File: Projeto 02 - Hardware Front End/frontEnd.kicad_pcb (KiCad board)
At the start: 2 copper layers, 75 x 50 mm, 22 parts, among them J1 Power_Supply, J2 Signal_Input, J3 MCU_Interface, U1 L78L12_TO92, U2 L79L12_TO92, U3 LM311

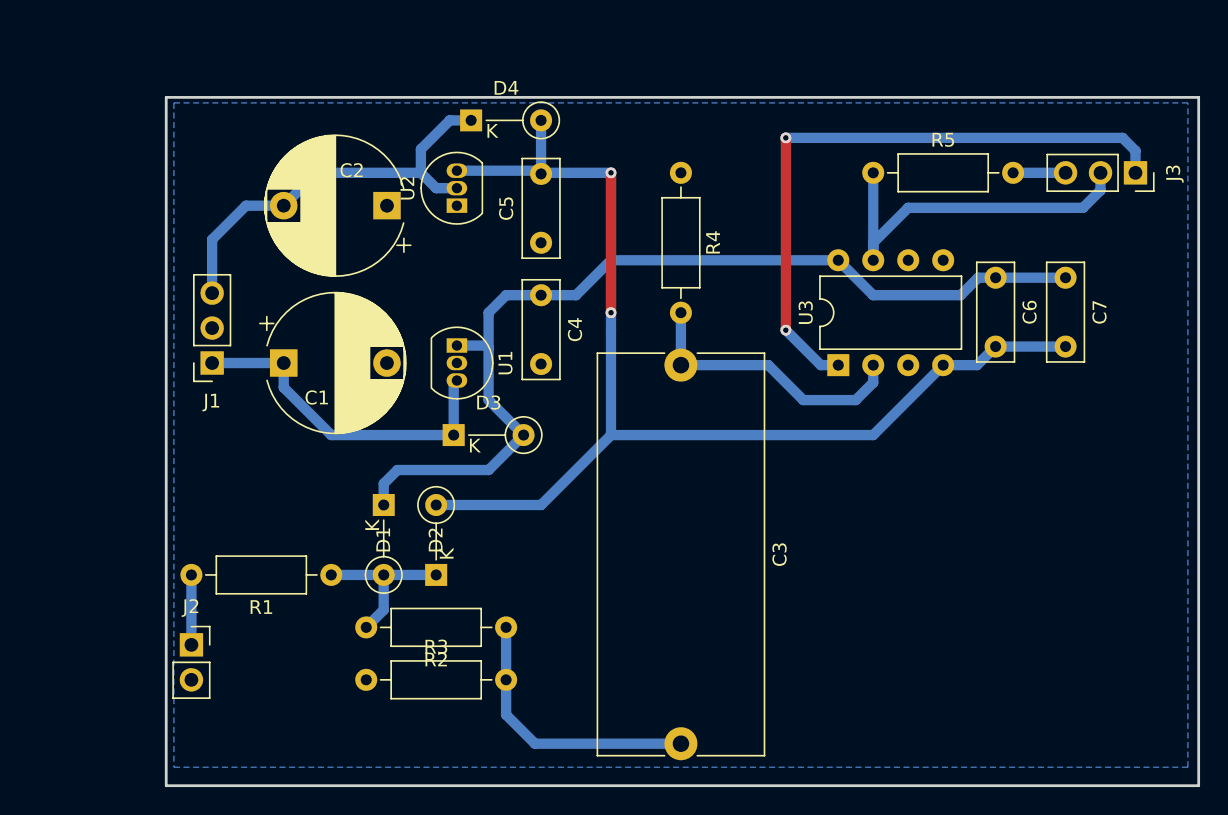
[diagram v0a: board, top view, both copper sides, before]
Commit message: Projeto CCS quase 100%
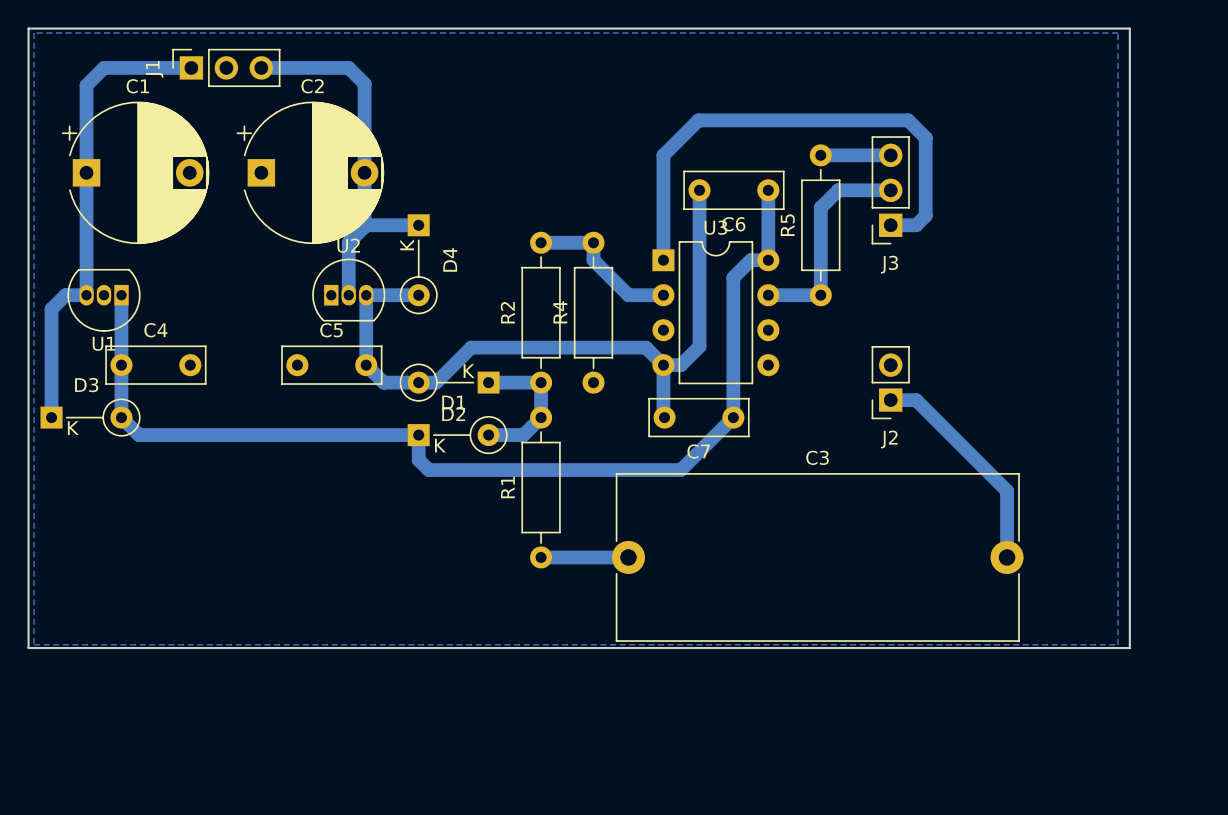
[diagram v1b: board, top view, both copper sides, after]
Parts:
- removed R3: 22k, Resistor_THT:R_Axial_DIN0207_L6.3mm_D2.5mm_P10.16mm_Horizontal
- R2: value 2.2k -> 68k
- moved J2 53.8 mm to (87.6, 47.0), turned to 180 degrees
- moved C4 30.9 mm to (31.8, 44.5), turned to 0 degrees
- moved D3 29.2 mm to (26.7, 48.3)
- moved C7 26.2 mm to (76.2, 48.3), turned to 180 degrees
- moved U1 24.6 mm to (31.8, 39.4), turned to 180 degrees
- moved J1 21.5 mm to (36.8, 22.9), turned to 90 degrees
- moved C1 19.9 mm to (29.2, 30.5)
- moved C5 19.8 mm to (44.5, 44.5), turned to 0 degrees
- moved J3 18.2 mm to (87.6, 34.3), turned to 180 degrees
- moved R2 18.0 mm to (62.2, 45.7), turned to 90 degrees
- moved C6 17.7 mm to (78.7, 31.8), turned to 180 degrees
- moved R4 16.5 mm to (66.0, 45.7), turned to 90 degrees
- moved R1 15.3 mm to (62.2, 58.4), turned to 90 degrees
- moved U3 14.8 mm to (71.1, 36.8), turned to 0 degrees
- moved C3 14.5 mm to (68.6, 58.4), turned to 0 degrees
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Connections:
- J2 pad 1: Net-(J2-Pad1) -> Net-(C3-Pad2)
- R1 pad 1: Net-(D1-Pad2) -> Net-(C3-Pad1)
- R1 pad 2: Net-(J2-Pad1) -> Net-(D1-Pad2)
- R2 pad 1: Net-(C3-Pad2) -> Net-(D1-Pad2)
- R2 pad 2: Net-(D1-Pad2) -> Net-(R2-Pad2)
- R4 pad 2: Net-(C3-Pad1) -> Net-(R2-Pad2)
- U3 pad 2: Net-(C3-Pad1) -> Net-(R2-Pad2)
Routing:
- net -12V: track 84.8 -> 51.0 mm, vias 2 -> 0
- net Net-(C3-Pad1): track 20.6 -> 6.35 mm
- net Net-(R2-Pad2): track 0.00 -> 11.2 mm
- net Net-(J3-Pad2): track 27.0 -> 15.8 mm
- net Net-(J3-Pad1): track 46.2 -> 36.7 mm, vias 2 -> 0
- net Net-(C1-Pad1): track 25.3 -> 34.2 mm
- net +12V: track 70.5 -> 75.9 mm
- net Net-(J2-Pad1): track 5.08 -> 0.00 mm
- net Net-(C3-Pad2): track 19.9 -> 16.0 mm
- net Net-(C2-Pad2): track 30.4 -> 27.8 mm
- net Net-(D1-Pad2): track 12.0 -> 10.7 mm
- net Net-(J3-Pad3): track 3.81 -> 5.08 mm
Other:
- board size 75 x 50 mm -> 80 x 45 mm
